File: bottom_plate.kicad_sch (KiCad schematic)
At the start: 25 parts, among them J42 Osc Out, J43 Conn_02x08_Odd_Even, J44 Conn_02x08_Odd_Even, J45 Conn_02x08_Odd_Even, J46 Conn_02x08_Odd_Even, J47 Conn_02x08_Odd_Even, J48 Select, J49 Select, J60 VCC, J61 VCC, J62 GND, J63 GND, J64 Conn_02x08_Odd_Even, J66 4017 Pins, J67 4017 Pins, J68 Conn_01x18, J73 Conn_02x22_Odd_Even, J74 Conn_02x22_Odd_Even, J75 Conn_02x22_Odd_Even, J76 Conn_02x22_Odd_Even, J77 Conn_02x22_Odd_Even, J78 Conn_02x22_Odd_Even, J79 Conn_02x22_Odd_Even, J80 Conn_02x22_Odd_Even, J81 Conn_02x22_Odd_Even

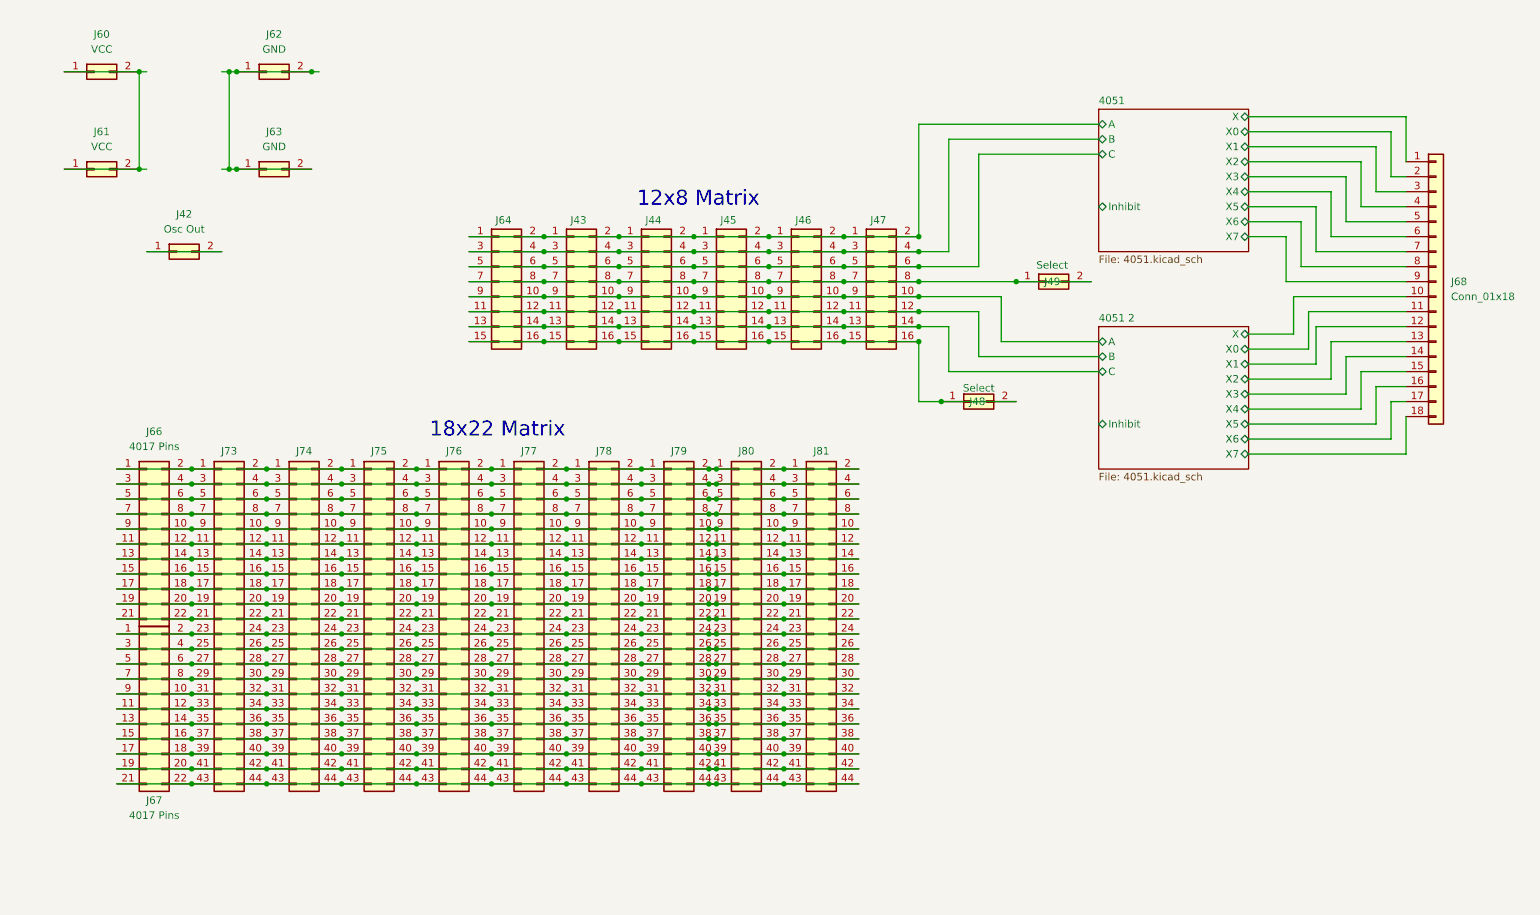
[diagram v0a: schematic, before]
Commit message: wip symmetric layout
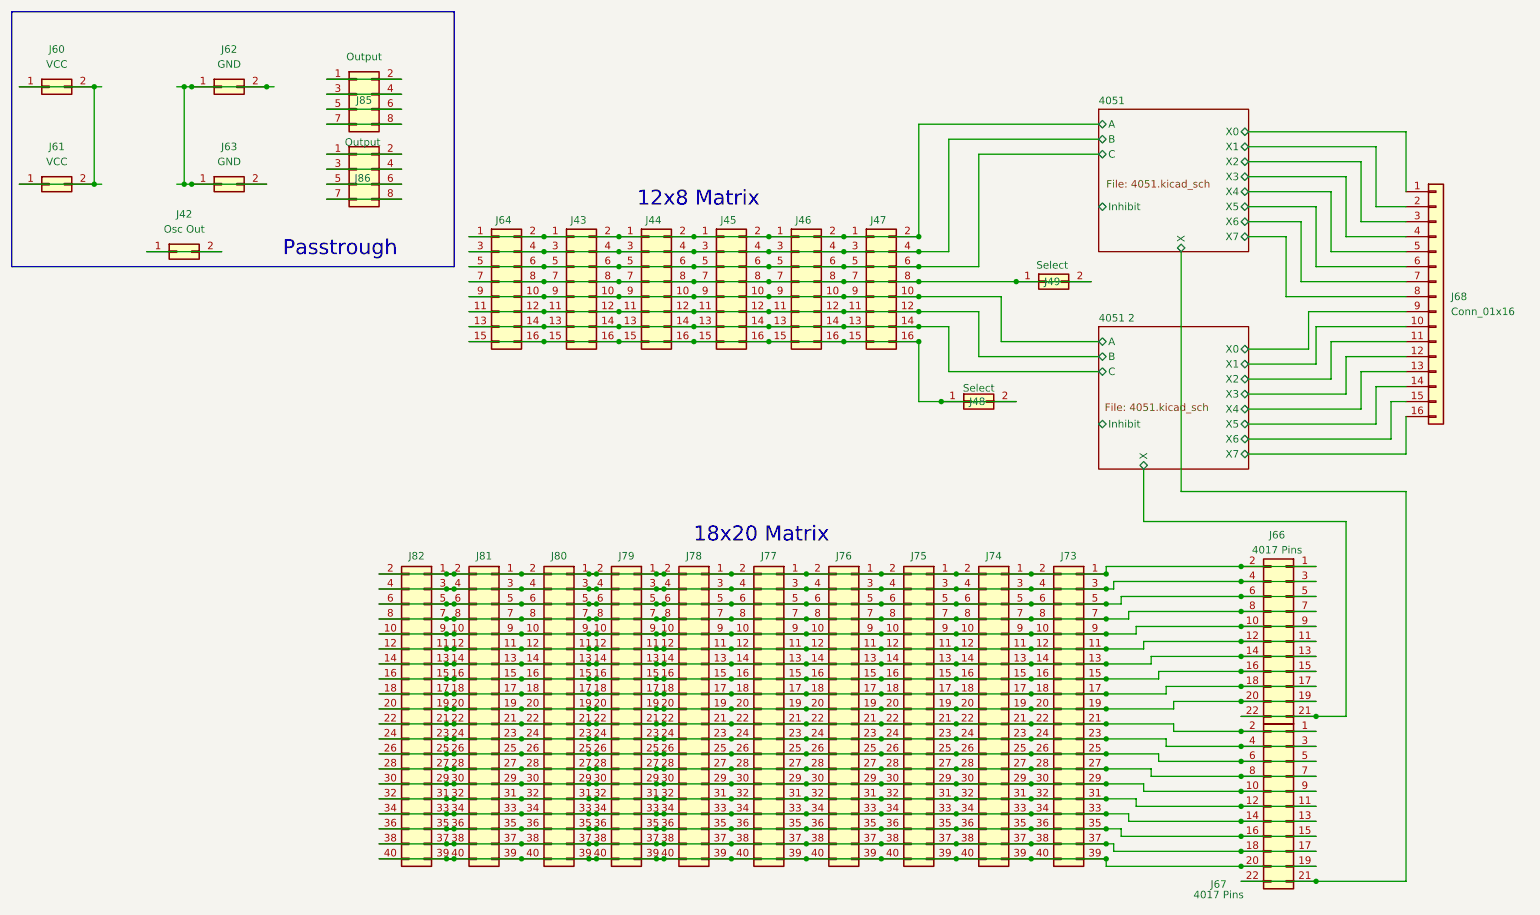
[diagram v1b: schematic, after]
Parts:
- removed J68: Conn_01x18, Connector_PinHeader_2.54mm:PinHeader_1x18_P2.54mm_Vertical, symbol Connector_Generic:Conn_01x18
- removed J73, J74, J75, J76, J77, J78, J79, J80, J81: Conn_02x22_Odd_Even, symbol Connector_Generic:Conn_02x22_Odd_Even
- added J68: Conn_01x16, Connector_PinSocket_2.54mm:PinSocket_1x16_P2.54mm_Vertical, symbol Connector_Generic:Conn_01x16
- added J73, J74, J75, J76, J77, J78, J79, J80, J81, J82: Conn_02x20_Odd_Even, Connector_PinHeader_2.54mm:PinHeader_2x20_P2.54mm_Vertical, symbol Connector_Generic:Conn_02x20_Odd_Even
- added J85, J86: Output, Connector_PinHeader_2.54mm:PinHeader_2x04_P2.54mm_Vertical, symbol Connector_Generic:Conn_02x04_Odd_Even
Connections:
- net 4051 2/X: now also J66.21 (Pin_21), J66.22 (Pin_22)
- net 4051 2/X0: now also J68.9 (Pin_9)
- net 4051 2/X1: now also J68.10 (Pin_10)
- net 4051 2/X2: now also J68.11 (Pin_11)
- net 4051 2/X3: now also J68.12 (Pin_12)
- net 4051 2/X4: now also J68.13 (Pin_13)
- net 4051 2/X5: now also J68.14 (Pin_14)
- net 4051 2/X6: now also J68.15 (Pin_15)
- net 4051 2/X7: now also J68.16 (Pin_16)
- net 4051/X: now also J67.21 (Pin_21), J67.22 (Pin_22)
- net 4051/X0: now also J68.1 (Pin_1)
- net 4051/X1: now also J68.2 (Pin_2)
- net 4051/X2: now also J68.3 (Pin_3)
- net 4051/X3: now also J68.4 (Pin_4)
- net 4051/X4: now also J68.5 (Pin_5)
- net 4051/X5: now also J68.6 (Pin_6)
- net 4051/X6: now also J68.7 (Pin_7)
- net 4051/X7: now also J68.8 (Pin_8)
- net at J66.1 (Pin_1), J66.2 (Pin_2): now also J73.1 (Pin_1), J73.2 (Pin_2), J74.1 (Pin_1), J74.2 (Pin_2), J75.1 (Pin_1), J75.2 (Pin_2), J76.1 (Pin_1), J76.2 (Pin_2), J77.1 (Pin_1), J77.2 (Pin_2), J78.1 (Pin_1), J78.2 (Pin_2), J79.1 (Pin_1), J79.2 (Pin_2), J80.1 (Pin_1), J80.2 (Pin_2), J81.1 (Pin_1), J81.2 (Pin_2), J82.1 (Pin_1), J82.2 (Pin_2)
- net at J66.10 (Pin_10), J66.9 (Pin_9): now also J73.10 (Pin_10), J73.9 (Pin_9), J74.10 (Pin_10), J74.9 (Pin_9), J75.10 (Pin_10), J75.9 (Pin_9), J76.10 (Pin_10), J76.9 (Pin_9), J77.10 (Pin_10), J77.9 (Pin_9), J78.10 (Pin_10), J78.9 (Pin_9), J79.10 (Pin_10), J79.9 (Pin_9), J80.10 (Pin_10), J80.9 (Pin_9), J81.10 (Pin_10), J81.9 (Pin_9), J82.10 (Pin_10), J82.9 (Pin_9)
- net at J66.11 (Pin_11), J66.12 (Pin_12): now also J73.11 (Pin_11), J73.12 (Pin_12), J74.11 (Pin_11), J74.12 (Pin_12), J75.11 (Pin_11), J75.12 (Pin_12), J76.11 (Pin_11), J76.12 (Pin_12), J77.11 (Pin_11), J77.12 (Pin_12), J78.11 (Pin_11), J78.12 (Pin_12), J79.11 (Pin_11), J79.12 (Pin_12), J80.11 (Pin_11), J80.12 (Pin_12), J81.11 (Pin_11), J81.12 (Pin_12), J82.11 (Pin_11), J82.12 (Pin_12)
- net at J66.13 (Pin_13), J66.14 (Pin_14): now also J73.13 (Pin_13), J73.14 (Pin_14), J74.13 (Pin_13), J74.14 (Pin_14), J75.13 (Pin_13), J75.14 (Pin_14), J76.13 (Pin_13), J76.14 (Pin_14), J77.13 (Pin_13), J77.14 (Pin_14), J78.13 (Pin_13), J78.14 (Pin_14), J79.13 (Pin_13), J79.14 (Pin_14), J80.13 (Pin_13), J80.14 (Pin_14), J81.13 (Pin_13), J81.14 (Pin_14), J82.13 (Pin_13), J82.14 (Pin_14)
- net at J66.15 (Pin_15), J66.16 (Pin_16): now also J73.15 (Pin_15), J73.16 (Pin_16), J74.15 (Pin_15), J74.16 (Pin_16), J75.15 (Pin_15), J75.16 (Pin_16), J76.15 (Pin_15), J76.16 (Pin_16), J77.15 (Pin_15), J77.16 (Pin_16), J78.15 (Pin_15), J78.16 (Pin_16), J79.15 (Pin_15), J79.16 (Pin_16), J80.15 (Pin_15), J80.16 (Pin_16), J81.15 (Pin_15), J81.16 (Pin_16), J82.15 (Pin_15), J82.16 (Pin_16)
- net at J66.17 (Pin_17), J66.18 (Pin_18): now also J73.17 (Pin_17), J73.18 (Pin_18), J74.17 (Pin_17), J74.18 (Pin_18), J75.17 (Pin_17), J75.18 (Pin_18), J76.17 (Pin_17), J76.18 (Pin_18), J77.17 (Pin_17), J77.18 (Pin_18), J78.17 (Pin_17), J78.18 (Pin_18), J79.17 (Pin_17), J79.18 (Pin_18), J80.17 (Pin_17), J80.18 (Pin_18), J81.17 (Pin_17), J81.18 (Pin_18), J82.17 (Pin_17), J82.18 (Pin_18)
- net at J66.19 (Pin_19), J66.20 (Pin_20): now also J73.19 (Pin_19), J73.20 (Pin_20), J74.19 (Pin_19), J74.20 (Pin_20), J75.19 (Pin_19), J75.20 (Pin_20), J76.19 (Pin_19), J76.20 (Pin_20), J77.19 (Pin_19), J77.20 (Pin_20), J78.19 (Pin_19), J78.20 (Pin_20), J79.19 (Pin_19), J79.20 (Pin_20), J80.19 (Pin_19), J80.20 (Pin_20), J81.19 (Pin_19), J81.20 (Pin_20), J82.19 (Pin_19), J82.20 (Pin_20)
- net at J67.1 (Pin_1), J67.2 (Pin_2): now also J73.21 (Pin_21), J73.22 (Pin_22), J74.21 (Pin_21), J74.22 (Pin_22), J75.21 (Pin_21), J75.22 (Pin_22), J76.21 (Pin_21), J76.22 (Pin_22), J77.21 (Pin_21), J77.22 (Pin_22), J78.21 (Pin_21), J78.22 (Pin_22), J79.21 (Pin_21), J79.22 (Pin_22), J80.21 (Pin_21), J80.22 (Pin_22), J81.21 (Pin_21), J81.22 (Pin_22), J82.21 (Pin_21), J82.22 (Pin_22)
- net at J67.3 (Pin_3), J67.4 (Pin_4): now also J73.23 (Pin_23), J73.24 (Pin_24), J74.23 (Pin_23), J74.24 (Pin_24), J75.23 (Pin_23), J75.24 (Pin_24), J76.23 (Pin_23), J76.24 (Pin_24), J77.23 (Pin_23), J77.24 (Pin_24), J78.23 (Pin_23), J78.24 (Pin_24), J79.23 (Pin_23), J79.24 (Pin_24), J80.23 (Pin_23), J80.24 (Pin_24), J81.23 (Pin_23), J81.24 (Pin_24), J82.23 (Pin_23), J82.24 (Pin_24)
- net at J67.5 (Pin_5), J67.6 (Pin_6): now also J73.25 (Pin_25), J73.26 (Pin_26), J74.25 (Pin_25), J74.26 (Pin_26), J75.25 (Pin_25), J75.26 (Pin_26), J76.25 (Pin_25), J76.26 (Pin_26), J77.25 (Pin_25), J77.26 (Pin_26), J78.25 (Pin_25), J78.26 (Pin_26), J79.25 (Pin_25), J79.26 (Pin_26), J80.25 (Pin_25), J80.26 (Pin_26), J81.25 (Pin_25), J81.26 (Pin_26), J82.25 (Pin_25), J82.26 (Pin_26)
- net at J67.7 (Pin_7), J67.8 (Pin_8): now also J73.27 (Pin_27), J73.28 (Pin_28), J74.27 (Pin_27), J74.28 (Pin_28), J75.27 (Pin_27), J75.28 (Pin_28), J76.27 (Pin_27), J76.28 (Pin_28), J77.27 (Pin_27), J77.28 (Pin_28), J78.27 (Pin_27), J78.28 (Pin_28), J79.27 (Pin_27), J79.28 (Pin_28), J80.27 (Pin_27), J80.28 (Pin_28), J81.27 (Pin_27), J81.28 (Pin_28), J82.27 (Pin_27), J82.28 (Pin_28)
- net at J66.3 (Pin_3), J66.4 (Pin_4): now also J73.3 (Pin_3), J73.4 (Pin_4), J74.3 (Pin_3), J74.4 (Pin_4), J75.3 (Pin_3), J75.4 (Pin_4), J76.3 (Pin_3), J76.4 (Pin_4), J77.3 (Pin_3), J77.4 (Pin_4), J78.3 (Pin_3), J78.4 (Pin_4), J79.3 (Pin_3), J79.4 (Pin_4), J80.3 (Pin_3), J80.4 (Pin_4), J81.3 (Pin_3), J81.4 (Pin_4), J82.3 (Pin_3), J82.4 (Pin_4)
- net at J67.10 (Pin_10), J67.9 (Pin_9): now also J73.29 (Pin_29), J73.30 (Pin_30), J74.29 (Pin_29), J74.30 (Pin_30), J75.29 (Pin_29), J75.30 (Pin_30), J76.29 (Pin_29), J76.30 (Pin_30), J77.29 (Pin_29), J77.30 (Pin_30), J78.29 (Pin_29), J78.30 (Pin_30), J79.29 (Pin_29), J79.30 (Pin_30), J80.29 (Pin_29), J80.30 (Pin_30), J81.29 (Pin_29), J81.30 (Pin_30), J82.29 (Pin_29), J82.30 (Pin_30)
- net at J67.11 (Pin_11), J67.12 (Pin_12): now also J73.31 (Pin_31), J73.32 (Pin_32), J74.31 (Pin_31), J74.32 (Pin_32), J75.31 (Pin_31), J75.32 (Pin_32), J76.31 (Pin_31), J76.32 (Pin_32), J77.31 (Pin_31), J77.32 (Pin_32), J78.31 (Pin_31), J78.32 (Pin_32), J79.31 (Pin_31), J79.32 (Pin_32), J80.31 (Pin_31), J80.32 (Pin_32), J81.31 (Pin_31), J81.32 (Pin_32), J82.31 (Pin_31), J82.32 (Pin_32)
- net at J67.13 (Pin_13), J67.14 (Pin_14): now also J73.33 (Pin_33), J73.34 (Pin_34), J74.33 (Pin_33), J74.34 (Pin_34), J75.33 (Pin_33), J75.34 (Pin_34), J76.33 (Pin_33), J76.34 (Pin_34), J77.33 (Pin_33), J77.34 (Pin_34), J78.33 (Pin_33), J78.34 (Pin_34), J79.33 (Pin_33), J79.34 (Pin_34), J80.33 (Pin_33), J80.34 (Pin_34), J81.33 (Pin_33), J81.34 (Pin_34), J82.33 (Pin_33), J82.34 (Pin_34)
- net at J67.15 (Pin_15), J67.16 (Pin_16): now also J73.35 (Pin_35), J73.36 (Pin_36), J74.35 (Pin_35), J74.36 (Pin_36), J75.35 (Pin_35), J75.36 (Pin_36), J76.35 (Pin_35), J76.36 (Pin_36), J77.35 (Pin_35), J77.36 (Pin_36), J78.35 (Pin_35), J78.36 (Pin_36), J79.35 (Pin_35), J79.36 (Pin_36), J80.35 (Pin_35), J80.36 (Pin_36), J81.35 (Pin_35), J81.36 (Pin_36), J82.35 (Pin_35), J82.36 (Pin_36)
- net at J67.17 (Pin_17), J67.18 (Pin_18): now also J73.37 (Pin_37), J73.38 (Pin_38), J74.37 (Pin_37), J74.38 (Pin_38), J75.37 (Pin_37), J75.38 (Pin_38), J76.37 (Pin_37), J76.38 (Pin_38), J77.37 (Pin_37), J77.38 (Pin_38), J78.37 (Pin_37), J78.38 (Pin_38), J79.37 (Pin_37), J79.38 (Pin_38), J80.37 (Pin_37), J80.38 (Pin_38), J81.37 (Pin_37), J81.38 (Pin_38), J82.37 (Pin_37), J82.38 (Pin_38)
- net at J67.19 (Pin_19), J67.20 (Pin_20): now also J73.39 (Pin_39), J73.40 (Pin_40), J74.39 (Pin_39), J74.40 (Pin_40), J75.39 (Pin_39), J75.40 (Pin_40), J76.39 (Pin_39), J76.40 (Pin_40), J77.39 (Pin_39), J77.40 (Pin_40), J78.39 (Pin_39), J78.40 (Pin_40), J79.39 (Pin_39), J79.40 (Pin_40), J80.39 (Pin_39), J80.40 (Pin_40), J81.39 (Pin_39), J81.40 (Pin_40), J82.39 (Pin_39), J82.40 (Pin_40)
- net at J66.5 (Pin_5), J66.6 (Pin_6): now also J73.5 (Pin_5), J73.6 (Pin_6), J74.5 (Pin_5), J74.6 (Pin_6), J75.5 (Pin_5), J75.6 (Pin_6), J76.5 (Pin_5), J76.6 (Pin_6), J77.5 (Pin_5), J77.6 (Pin_6), J78.5 (Pin_5), J78.6 (Pin_6), J79.5 (Pin_5), J79.6 (Pin_6), J80.5 (Pin_5), J80.6 (Pin_6), J81.5 (Pin_5), J81.6 (Pin_6), J82.5 (Pin_5), J82.6 (Pin_6)
- net at J66.7 (Pin_7), J66.8 (Pin_8): now also J73.7 (Pin_7), J73.8 (Pin_8), J74.7 (Pin_7), J74.8 (Pin_8), J75.7 (Pin_7), J75.8 (Pin_8), J76.7 (Pin_7), J76.8 (Pin_8), J77.7 (Pin_7), J77.8 (Pin_8), J78.7 (Pin_7), J78.8 (Pin_8), J79.7 (Pin_7), J79.8 (Pin_8), J80.7 (Pin_7), J80.8 (Pin_8), J81.7 (Pin_7), J81.8 (Pin_8), J82.7 (Pin_7), J82.8 (Pin_8)
- new net: J86.1 (Pin_1), J86.2 (Pin_2)
- new net: J86.3 (Pin_3), J86.4 (Pin_4)
- new net: J86.5 (Pin_5), J86.6 (Pin_6)
- new net: J86.7 (Pin_7), J86.8 (Pin_8)
- new net: J85.1 (Pin_1), J85.2 (Pin_2)
- new net: J85.3 (Pin_3), J85.4 (Pin_4)
- new net: J85.5 (Pin_5), J85.6 (Pin_6)
- new net: J85.7 (Pin_7), J85.8 (Pin_8)
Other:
- note added: "18x20 Matrix"
- note added: "Passtrough"
- note removed: "18x22 Matrix"
- moved on the sheet: J60, J61, J62, J63, J66, J67
